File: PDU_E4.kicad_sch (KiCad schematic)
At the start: 7 parts, among them K1 EV200, K2 SVC50, K3 EV200, K4 SVC50, K5 EV200

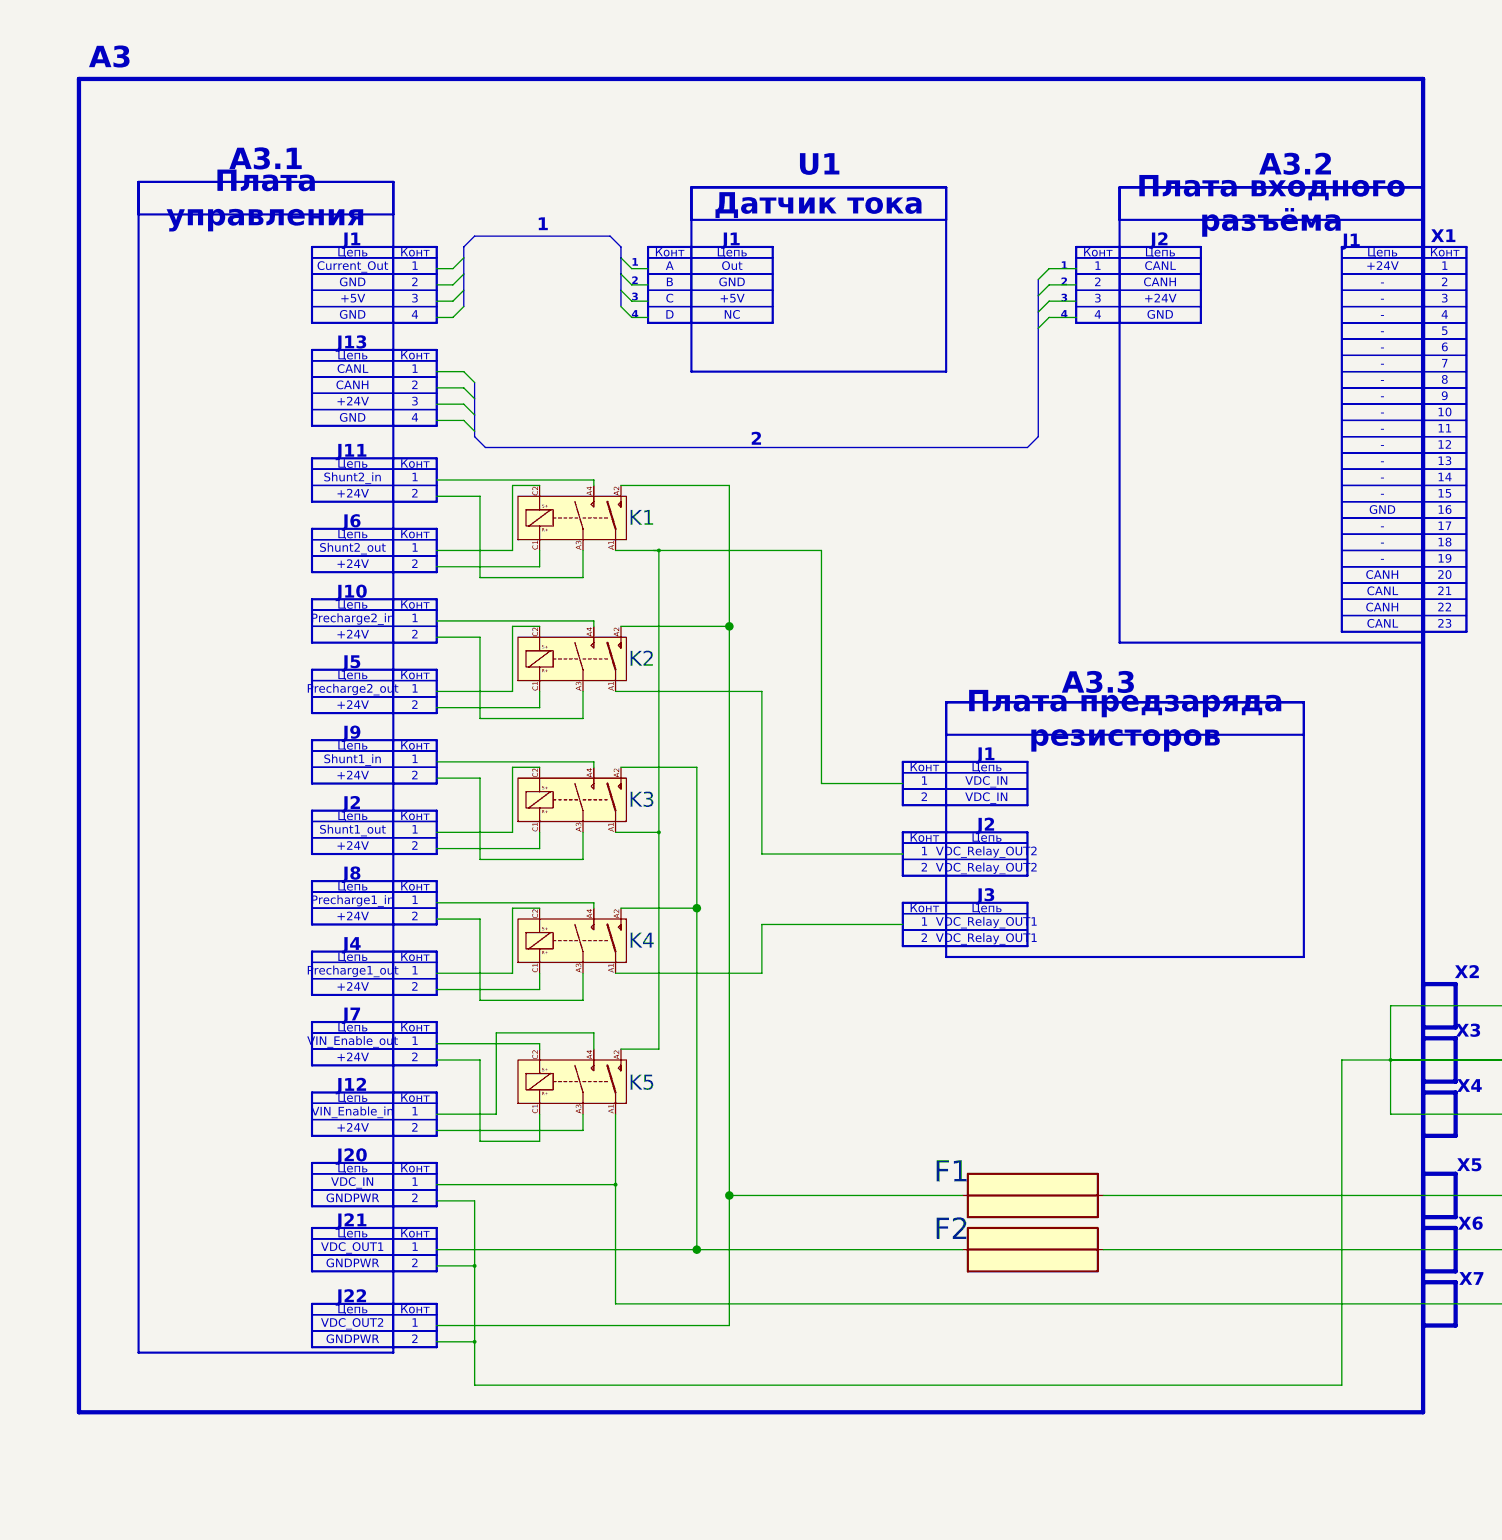
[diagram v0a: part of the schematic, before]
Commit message: VER1: добавил новую версию схемы
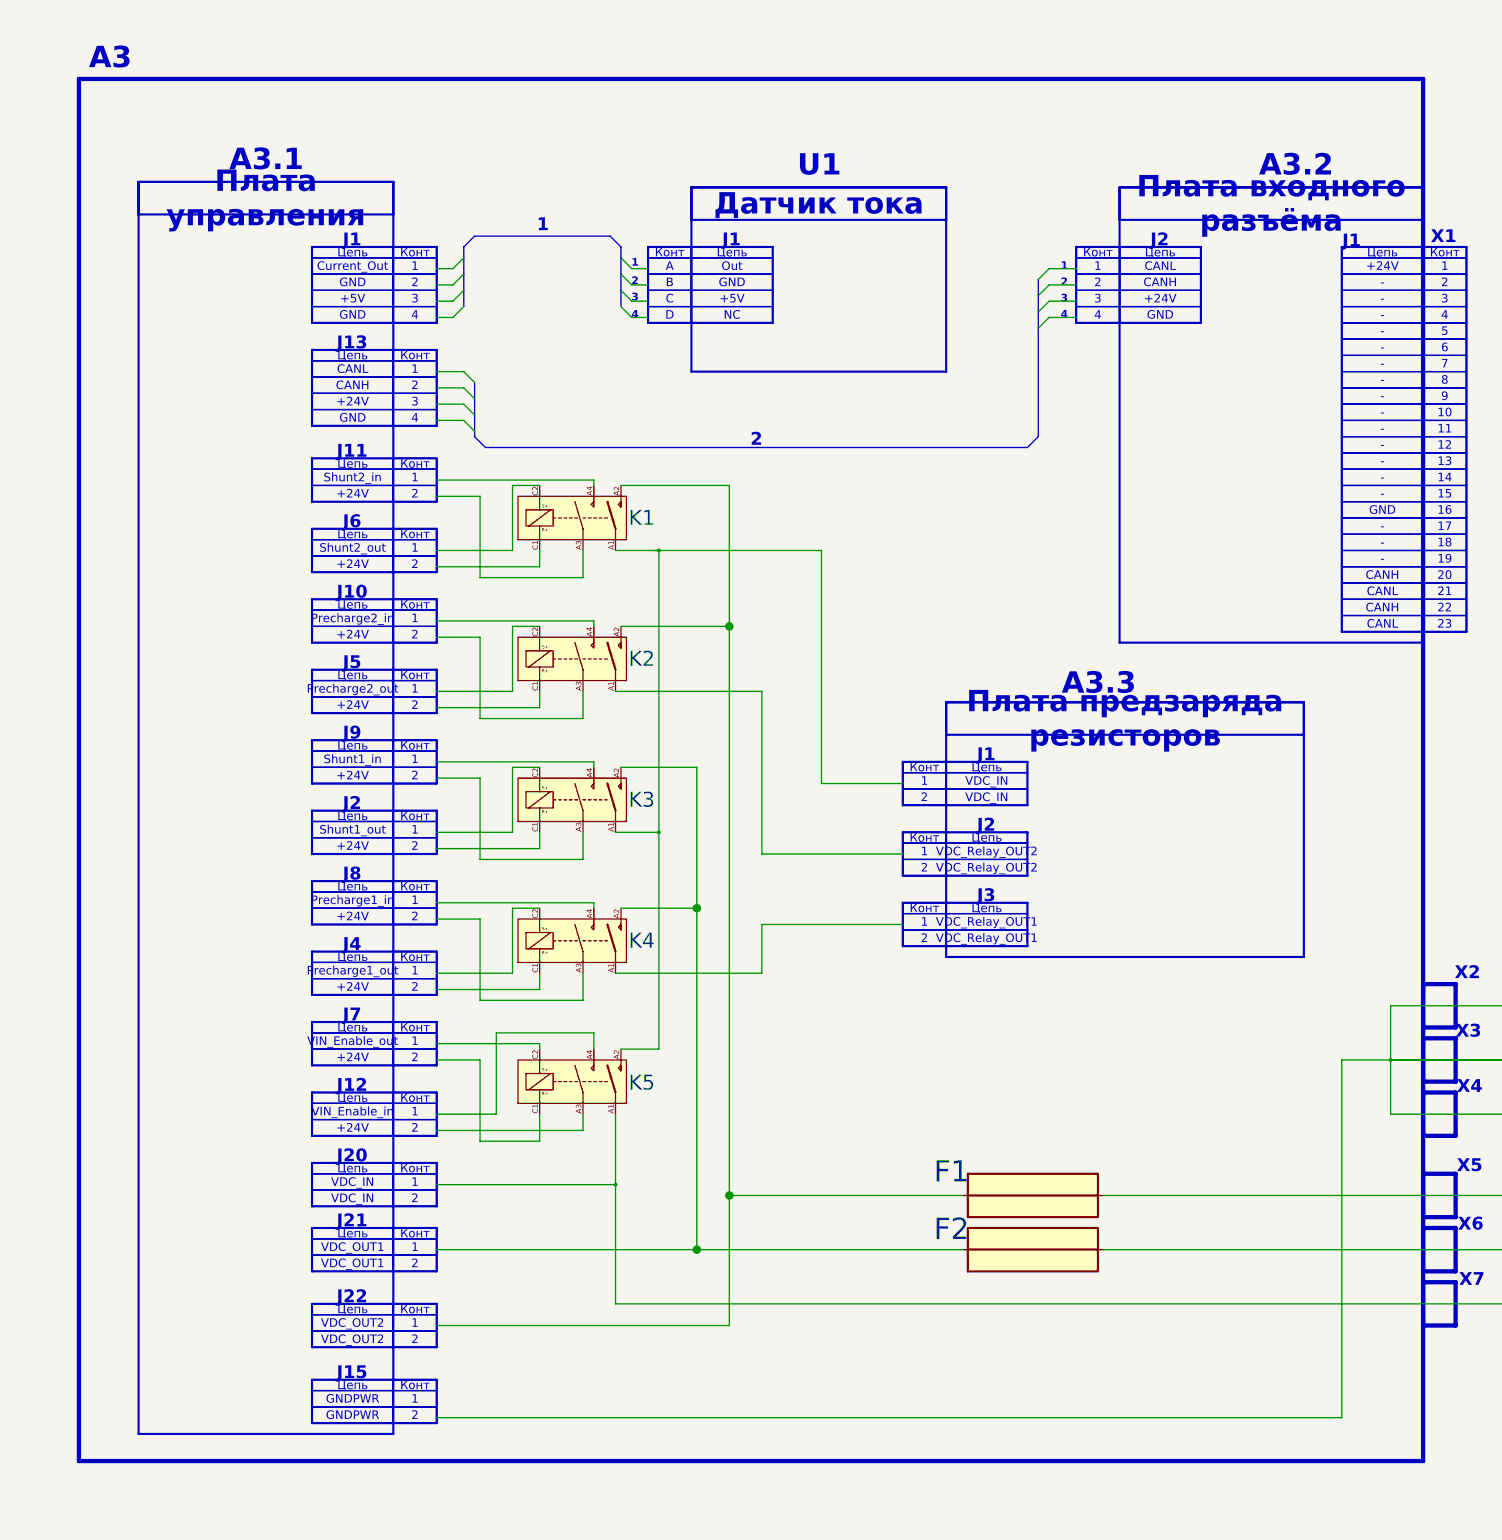
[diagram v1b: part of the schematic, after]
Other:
- note added: "J15"
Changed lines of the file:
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@@
 		(title "Блок распределения питания силовой")
 		(date "2025-06-02")
-		(comment 1 "НВЦТ.0001.0400.100 Э4")
+		(comment 1 "НВЦТ.0001.0400.100_v1. Э4")
 		(comment 2 "Филатов А.С.")
 		(comment 3 "Сизякин А.В.")
@@
 	(rectangle
 		(start 60.96 71.12)
-		(end 120.65 345.44)
+		(end 120.65 364.49)
 		(stroke
 			(width 0.5)
@@
 	)
 	(rectangle
+		(start 101.6 351.79)
+		(end 130.81 361.95)
+		(stroke
+			(width 0.5)
+			(type default)
+		)
+		(fill
+			(type none)
+		)
+	)
+	(rectangle
 		(start 240.03 223.52)
 		(end 269.24 233.68)
@@
 	)
 	(rectangle
+		(start 120.65 351.79)
+		(end 130.81 361.95)
+		(stroke
+			(width 0)
+			(type solid)
+		)
+		(fill
+			(type color)
+			(color 194 194 194 1)
+		)
+	)
+	(rectangle
 		(start 280.67 86.36)
 		(end 290.83 104.14)
@@
 	(rectangle
 		(start 46.99 46.99)
-		(end 361.95 359.41)
+		(end 361.95 370.84)
 		(stroke
 			(width 1)
@@
 		)
 	)
+	(text "J15"
+		(exclude_from_sim no)
+		(at 110.998 350.266 0)
+		(effects
+			(font
+				(size 3 3)
+				(thickness 0.6)
+				(bold yes)
+			)
+		)
+	)
 	(text "X5"
 		(exclude_from_sim no)
@@
 		)
 	)
+	(text_box "GNDPWR"
+		(exclude_from_sim no)
+		(at 101.6 358.14 0)
+		(size 19.05 3.81)
+		(margins 1.5 1.5 1.5 1.5)
+		(stroke
+			(width 0)
+			(type solid)
+		)
+		(fill
+			(type none)
+		)
+		(effects
+			(font
+				(size 2 2)
+			)
+		)
+	)
 	(text_box "GND"
 		(exclude_from_sim no)
@@
 		)
 	)
-	(text_box "GNDPWR"
+	(text_box "VDC_OUT2"
 		(exclude_from_sim no)
 		(at 101.6 340.36 0)
@@
 		)
 	)
-	(text_box "GNDPWR"
+	(text_box "VDC_OUT1"
 		(exclude_from_sim no)
 		(at 101.6 322.58 0)
@@
 		)
 	)
+	(text_box "GNDPWR"
+		(exclude_from_sim no)
+		(at 101.6 354.33 0)
+		(size 19.05 3.81)
+		(margins 1.5 1.5 1.5 1.5)
+		(stroke
+			(width 0)
+			(type solid)
+		)
+		(fill
+			(type none)
+		)
+		(effects
+			(font
+				(size 2 2)
+			)
+		)
+	)
 	(text_box "CANL"
 		(exclude_from_sim no)
@@
 	(text_box "Конт"
 		(exclude_from_sim no)
+		(at 120.65 351.79 0)
+		(size 10.16 2.54)
+		(margins 1.5 1.5 1.5 1.5)
+		(stroke
+			(width 0)
+			(type default)
+		)
+		(fill
+			(type none)
+		)
+		(effects
+			(font
+				(size 2 2)
+			)
+		)
+	)
+	(text_box "Конт"
+		(exclude_from_sim no)
 		(at 240.03 240.03 0)
 		(size 10.16 2.54)
@@
 		)
 	)
+	(text_box "2\n"
+		(exclude_from_sim no)
+		(at 120.65 358.14 0)
+		(size 10.16 3.81)
+		(margins 1.5 1.5 1.5 1.5)
+		(stroke
+			(width 0)
+			(type default)
+		)
+		(fill
+			(type none)
+		)
+		(effects
+			(font
+				(size 2 2)
+			)
+		)
+	)
 	(text_box "K1,K3,K5"
 		(exclude_from_sim no)
@@
 		)
 	)
-	(text_box "GNDPWR"
+	(text_box "VDC_IN"
 		(exclude_from_sim no)
 		(at 101.6 307.34 0)
@@
 		)
 	)
+	(text_box "Цепь"
+		(exclude_from_sim no)
+		(at 101.6 351.79 0)
+		(size 19.05 2.54)
+		(margins 1.5 1.5 1.5 1.5)
+		(stroke
+			(width 0)
+			(type default)
+		)
+		(fill
+			(type none)
+		)
+		(effects
+			(font
+				(size 2 2)
+			)
+		)
+	)
 	(text_box "2\n"
 		(exclude_from_sim no)
@@
 		)
 	)
+	(text_box "1"
+		(exclude_from_sim no)
+		(at 120.65 354.33 0)
+		(size 10.16 3.81)
+		(margins 1.5 1.5 1.5 1.5)
+		(stroke
+			(width 0)
+			(type default)
+		)
+		(fill
+			(type none)
+		)
+		(effects
+			(font
+				(size 2 2)
+			)
+		)
+	)
 	(text_box "VDC_Relay_OUT2"
 		(exclude_from_sim no)
@@
 	)
 	(junction
-		(at 139.7 342.9)
-		(diameter 0)
-		(color 0 0 0 0)
-	)
-	(junction
 		(at 172.72 306.07)
 		(diameter 0)
@@
 	)
 	(junction
-		(at 139.7 325.12)
-		(diameter 0)
-		(color 0 0 0 0)
-	)
-	(junction
 		(at 182.88 157.48)
 		(diameter 0)
@@
 	(wire
 		(pts
-			(xy 130.81 325.12) (xy 139.7 325.12)
-		)
-		(stroke
-			(width 0)
-			(type default)
-		)
-	)
-	(wire
-		(pts
 			(xy 154.94 194.31) (xy 154.94 190.5)
 		)
@@
 	(wire
 		(pts
-			(xy 342.9 353.06) (xy 139.7 353.06)
-		)
-		(stroke
-			(width 0)
-			(type default)
-		)
-	)
-	(wire
-		(pts
 			(xy 130.81 140.97) (xy 167.64 140.97)
 		)
@@
 	(wire
 		(pts
-			(xy 139.7 325.12) (xy 139.7 342.9)
+			(xy 342.9 276.86) (xy 342.9 360.68)
 		)
 		(stroke
@@
 	(wire
 		(pts
-			(xy 342.9 276.86) (xy 342.9 353.06)
+			(xy 130.81 360.68) (xy 342.9 360.68)
 		)
 		(stroke
@@
 		)
 	)
-	(wire
-		(pts
-			(xy 130.81 342.9) (xy 139.7 342.9)
-		)
-		(stroke
-			(width 0)
-			(type default)
-		)
-	)
 	(bus
 		(pts
@@
 	(wire
 		(pts
-			(xy 139.7 325.12) (xy 139.7 309.88)
-		)
-		(stroke
-			(width 0)
-			(type default)
-		)
-	)
-	(wire
-		(pts
 			(xy 148.59 256.54) (xy 148.59 241.3)
 		)
@@
 	(wire
 		(pts
-			(xy 130.81 309.88) (xy 139.7 309.88)
-		)
-		(stroke
-			(width 0)
-			(type default)
-		)
-	)
-	(wire
-		(pts
 			(xy 180.34 95.25) (xy 176.53 95.25)
 		)
@@
 		)
 		(stroke
-			(width 0)
-			(type default)
-		)
-	)
-	(wire
-		(pts
-			(xy 139.7 353.06) (xy 139.7 342.9)
-		)
-		(stroke

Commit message: VER1: изменил схему
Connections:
- net VDC_IN: now also K1.A1, K3.A1; no longer K5.A1
- new net GNDPWR_OUT: K5.A2
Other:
- note added: "НВЦТ.0001.0400.100_v1"
- note removed: "НВЦТ.0001.0400.100"
